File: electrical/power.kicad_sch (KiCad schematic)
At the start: 63 parts

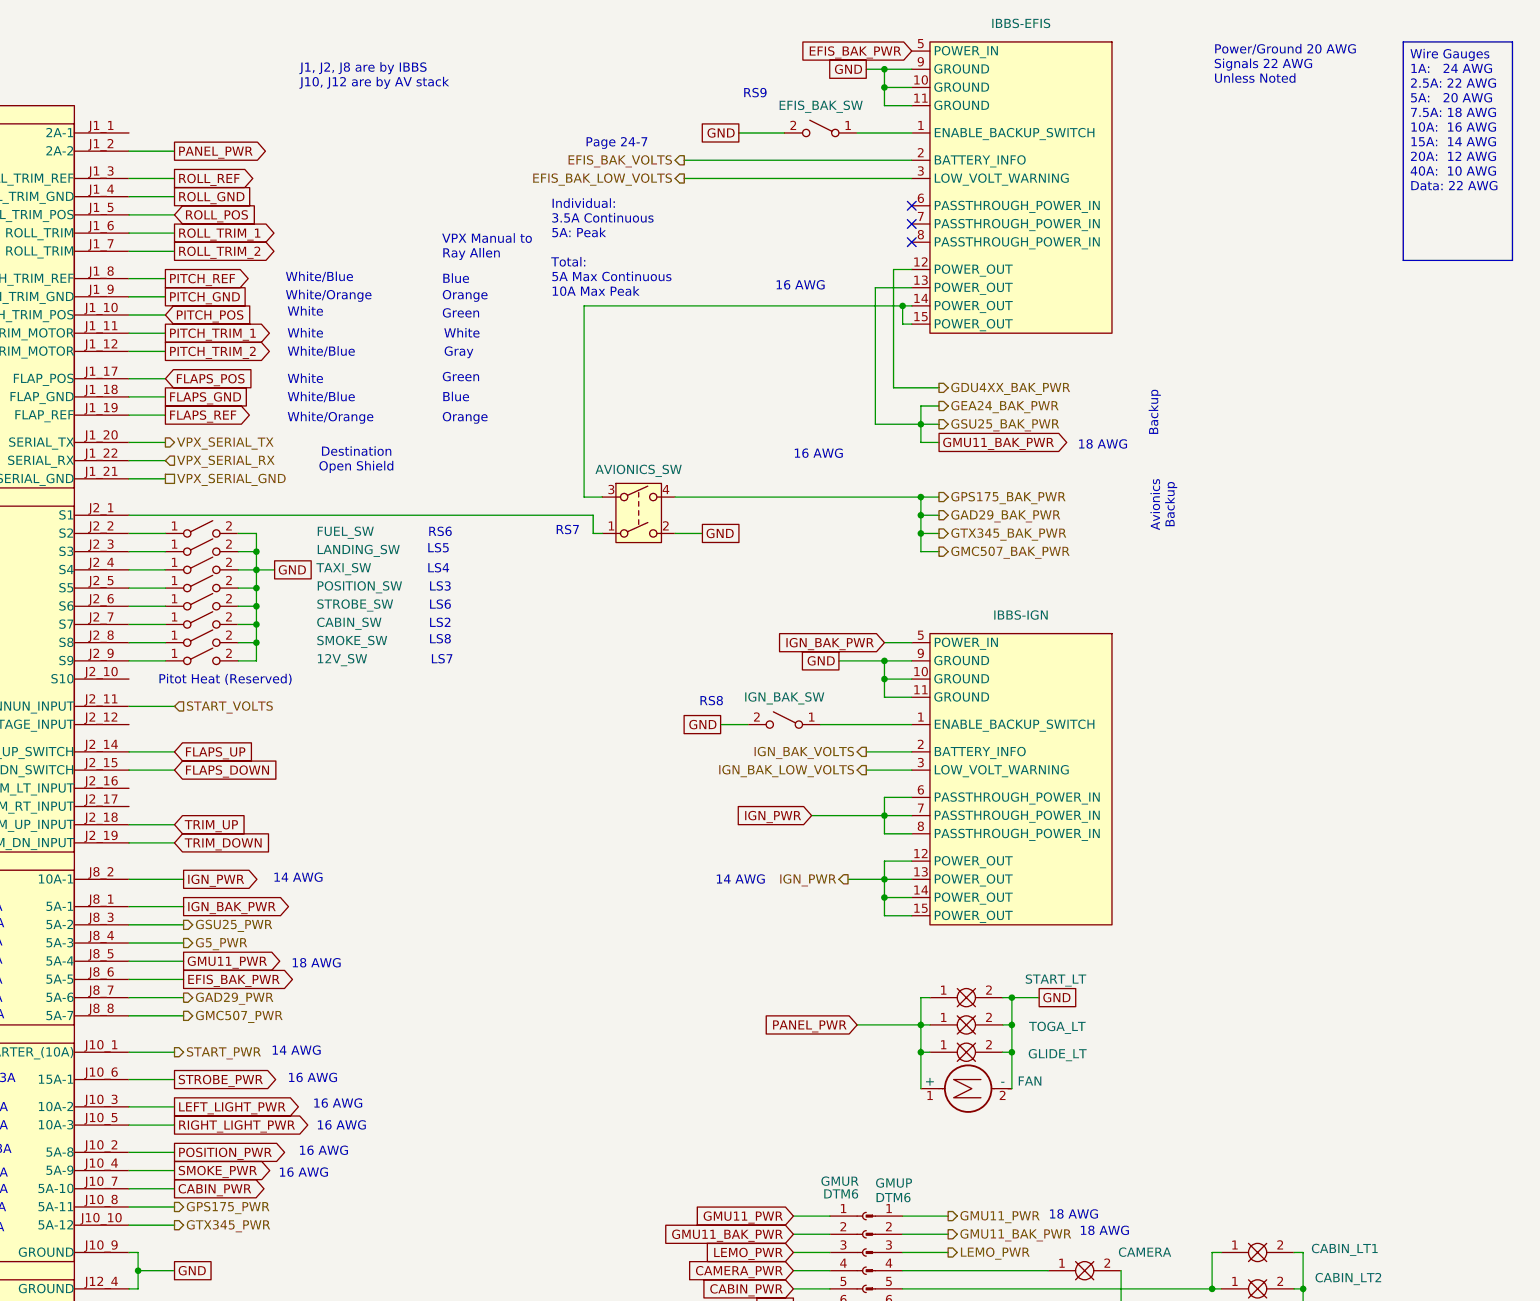
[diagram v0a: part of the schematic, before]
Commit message: Added lighting bus
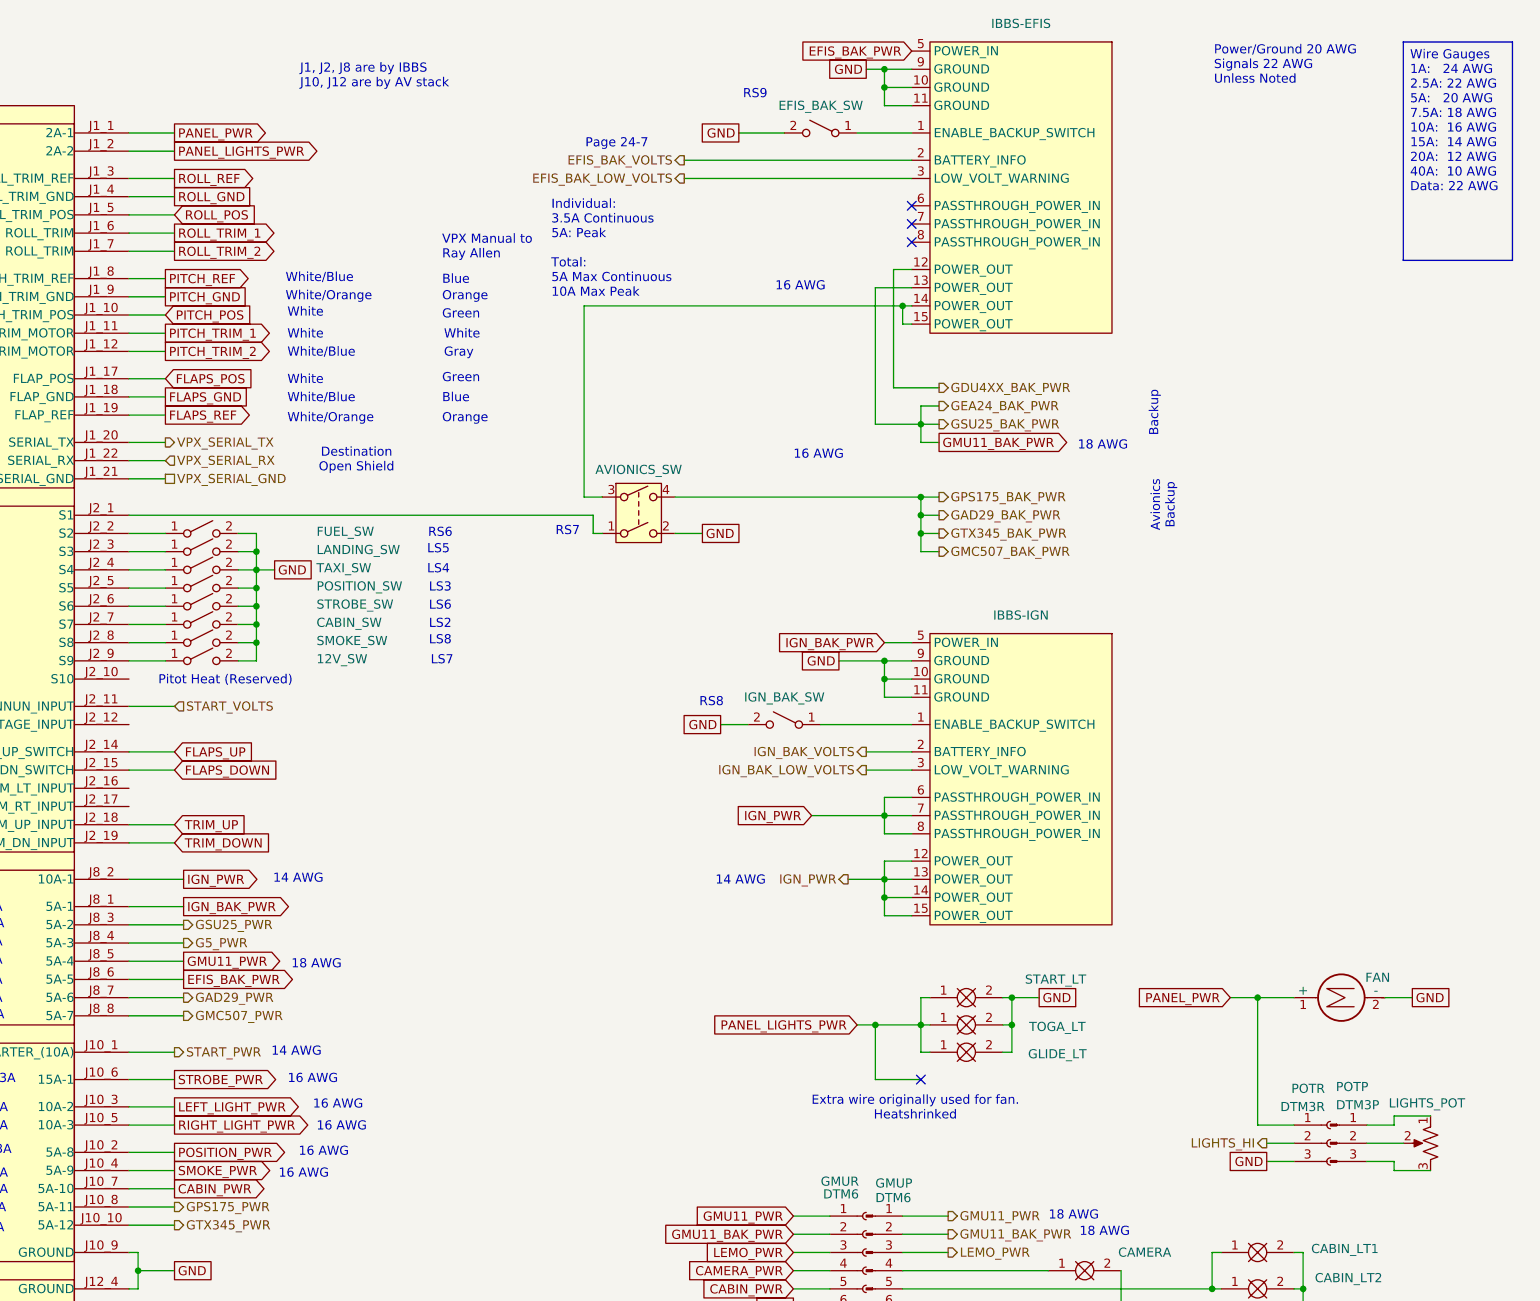
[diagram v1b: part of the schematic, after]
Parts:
- added LIGHTS_POT: R_Potentiometer_US, symbol Device:R_Potentiometer_US
- added POTP: DTM3P, symbol Connector:Conn_01x03_Pin
- added POTR: DTM3R, symbol Connector:Conn_01x03_Socket
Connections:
- net GND: now also POTR.3 (Pin_3)
- net PANEL_PWR: now also VPX.J1_1 (2A-1), POTR.1 (Pin_1); no longer GLIDE_LT.1, START_LT.1, TOGA_LT.1, VPX.J1_2 (2A-2)
- new net: LIGHTS_POT.1, POTP.1 (Pin_1)
- new net: LIGHTS_POT.2, POTP.2 (Pin_2)
- new net: LIGHTS_POT.3, POTP.3 (Pin_3)
- new net LIGHTS_HI: POTR.2 (Pin_2)
- new net PANEL_LIGHTS_PWR: GLIDE_LT.1, START_LT.1, TOGA_LT.1, VPX.J1_2 (2A-2)
- no-connect marks 7 -> 8
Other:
- note added: "Extra wire originally used for fan. Heatshrinked"
- moved on the sheet: FAN
